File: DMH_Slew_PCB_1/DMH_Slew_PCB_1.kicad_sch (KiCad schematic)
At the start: 0 parts

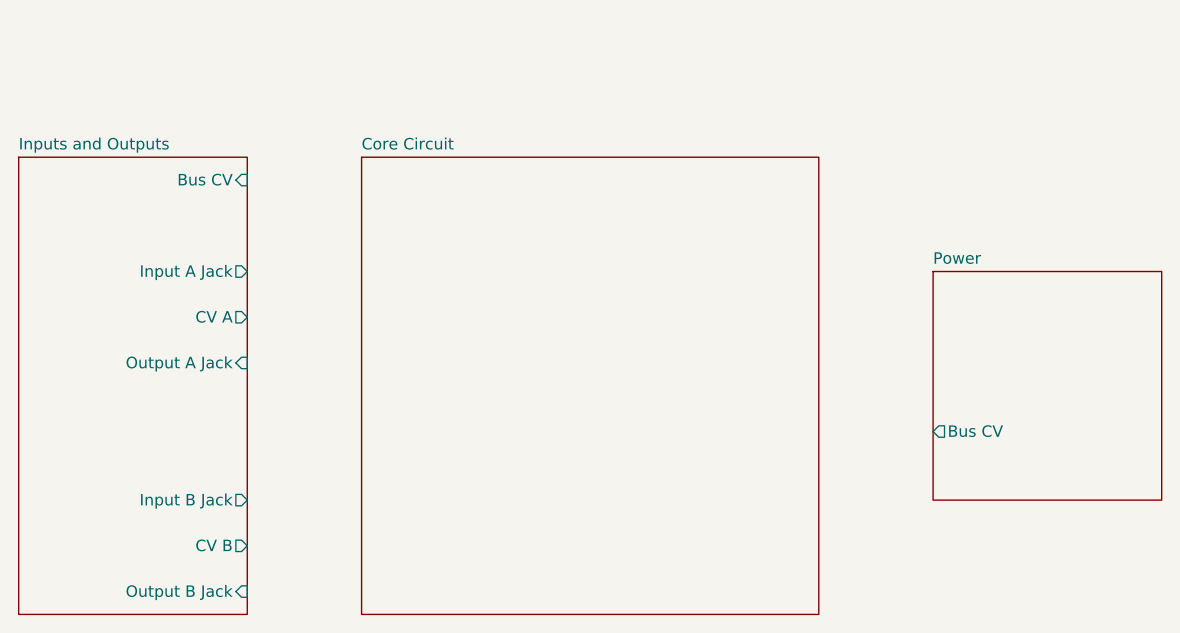
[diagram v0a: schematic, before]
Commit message: Schematic design in progress
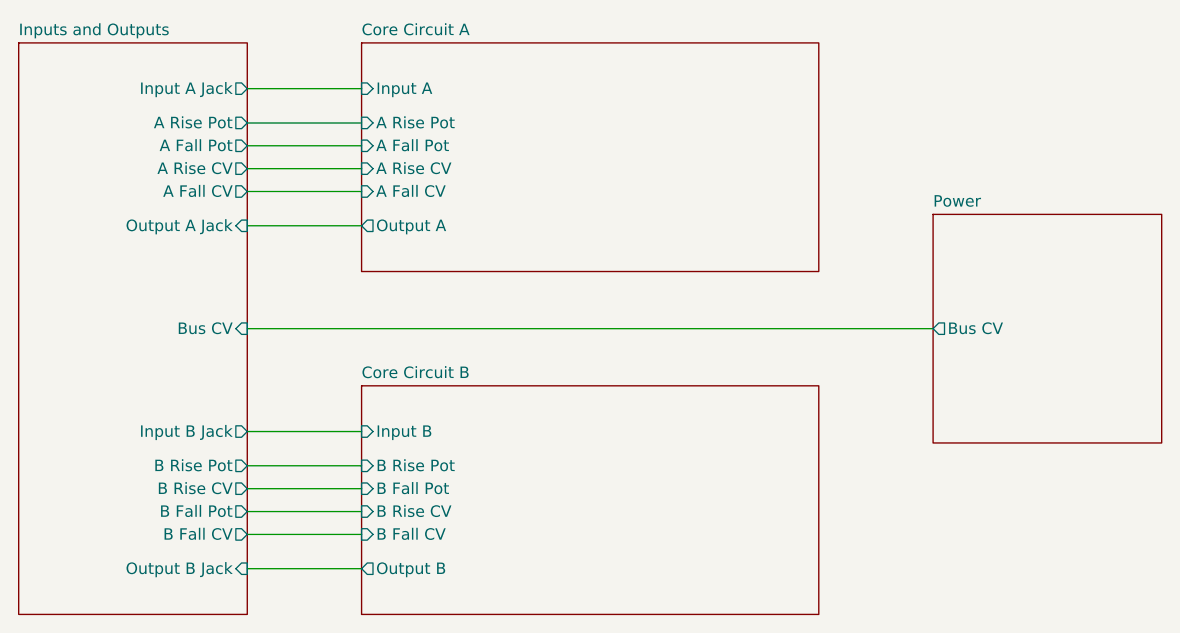
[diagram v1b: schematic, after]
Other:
- sheet Core Circuit renamed Core Circuit A
- added sheet Core Circuit B (Core_Circuit_B.kicad_sch)
- sheet Core Circuit A: file Core_Circuit.kicad_sch -> Core_Circuit_A.kicad_sch
- sheet Core Circuit A ports: added A Fall CV, A Fall Pot, A Rise CV, A Rise Pot, Input A, Output A; removed none
- sheet Inputs and Outputs ports: added A Fall CV, A Fall Pot, A Rise CV, A Rise Pot, B Fall CV, B Fall Pot, B Rise CV, B Rise Pot; removed CV A, CV B
